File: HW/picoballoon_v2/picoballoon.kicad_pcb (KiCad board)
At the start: 4 copper layers, 43 x 45 mm, 88 parts, among them IC1 MCXC141VLH, J1 EXT_DEBUGGER, J2 Conn_01x02, J3 Conn_Coaxial, Q1 PMOS, U1 Si4461, U2 MPL3115A2, U4 MCP9802, U5 MAX-M10S, U6 OPA333xxDBV, Y1 30M

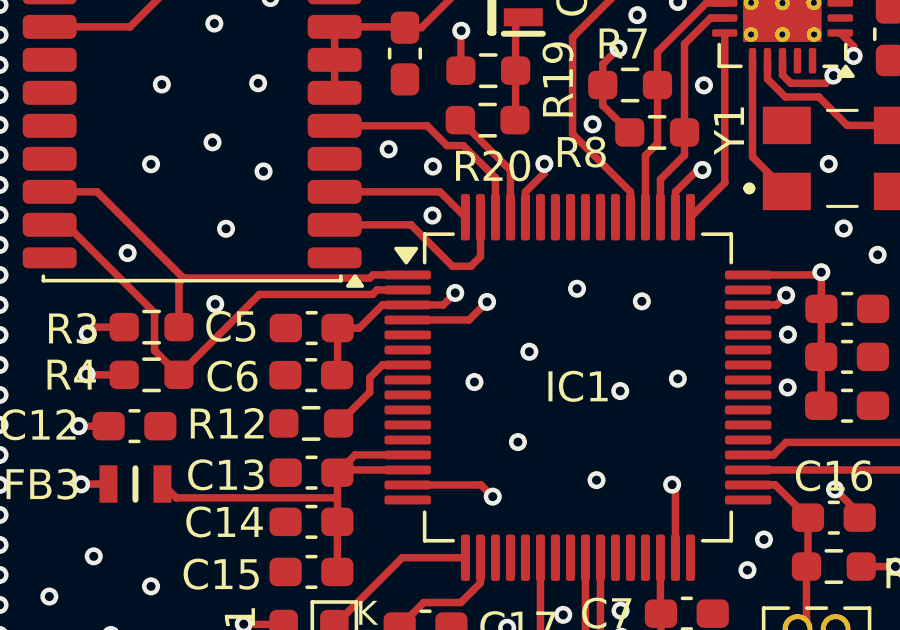
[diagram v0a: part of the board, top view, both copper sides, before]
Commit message: GND fix
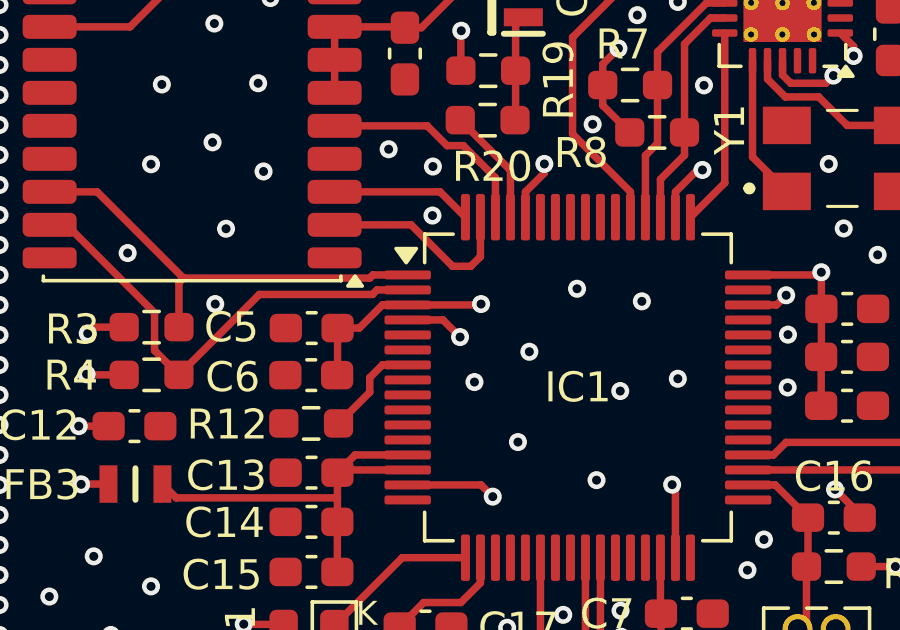
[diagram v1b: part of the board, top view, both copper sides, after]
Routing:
- net GND: track 16.5 -> 15.6 mm
- net +3.3V: track 75.7 -> 76.4 mm
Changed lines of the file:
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@@
 			)
 			(layer "F.SilkS")
+			(net 146735712)
 		)
 		(fp_line
@@
 	)
 	(segment
-		(start 135.14 102.31)
-		(end 135.74 101.71)
+		(start 133.095 102.31)
+		(end 134.27 102.31)
 		(width 0.25)
 		(layer "F.Cu")
@@
 	)
 	(segment
-		(start 133.095 102.31)
-		(end 135.14 102.31)
+		(start 142.02 110.235)
+		(end 142.02 107.91)
 		(width 0.25)
 		(layer "F.Cu")
@@
 	)
 	(segment
-		(start 142.02 110.235)
-		(end 142.02 107.91)
+		(start 134.27 102.31)
+		(end 134.84 102.88)
 		(width 0.25)
 		(layer "F.Cu")
@@
 	)
 	(via
-		(at 135.74 101.71)
+		(at 134.84 102.88)
 		(size 0.6)
 		(drill 0.3)
@@
 	)
 	(segment
-		(start 134.28 101.81)
-		(end 134.68 101.41)
-		(width 0.25)
-		(layer "F.Cu")
-		(net 5)
-	)
-	(segment
 		(start 145.58875 89.82)
 		(end 145.58875 88.955)
@@
 	)
 	(segment
+		(start 135.51 101.81)
+		(end 135.54 101.78)
+		(width 0.25)
+		(layer "F.Cu")
+		(net 5)
+	)
+	(segment
 		(start 149.98 117.9525)
 		(end 149.98 119.07)
@@
 	)
 	(segment
+		(start 133.095 101.81)
+		(end 135.51 101.81)
+		(width 0.25)
+		(layer "F.Cu")
+		(net 5)
+	)
+	(segment
 		(start 148.98 125.12)
 		(end 151.0225 125.12)
@@
 	)
 	(segment
-		(start 133.095 101.81)
-		(end 134.28 101.81)
-		(width 0.25)
-		(layer "F.Cu")
-		(net 5)
-	)
-	(segment
 		(start 154.665 115.24)
 		(end 154.78 115.355)
@@
 	)
 	(via
-		(at 134.68 101.41)
+		(at 135.54 101.78)
 		(size 0.6)
 		(drill 0.3)
